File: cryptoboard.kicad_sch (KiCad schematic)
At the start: 27 parts, among them J1 USB_A, J2 BOOT, J3 SWD, SW1 SW_Push, U1 STM32F103C8Tx, U2 LM317_SOT-223-3.3V

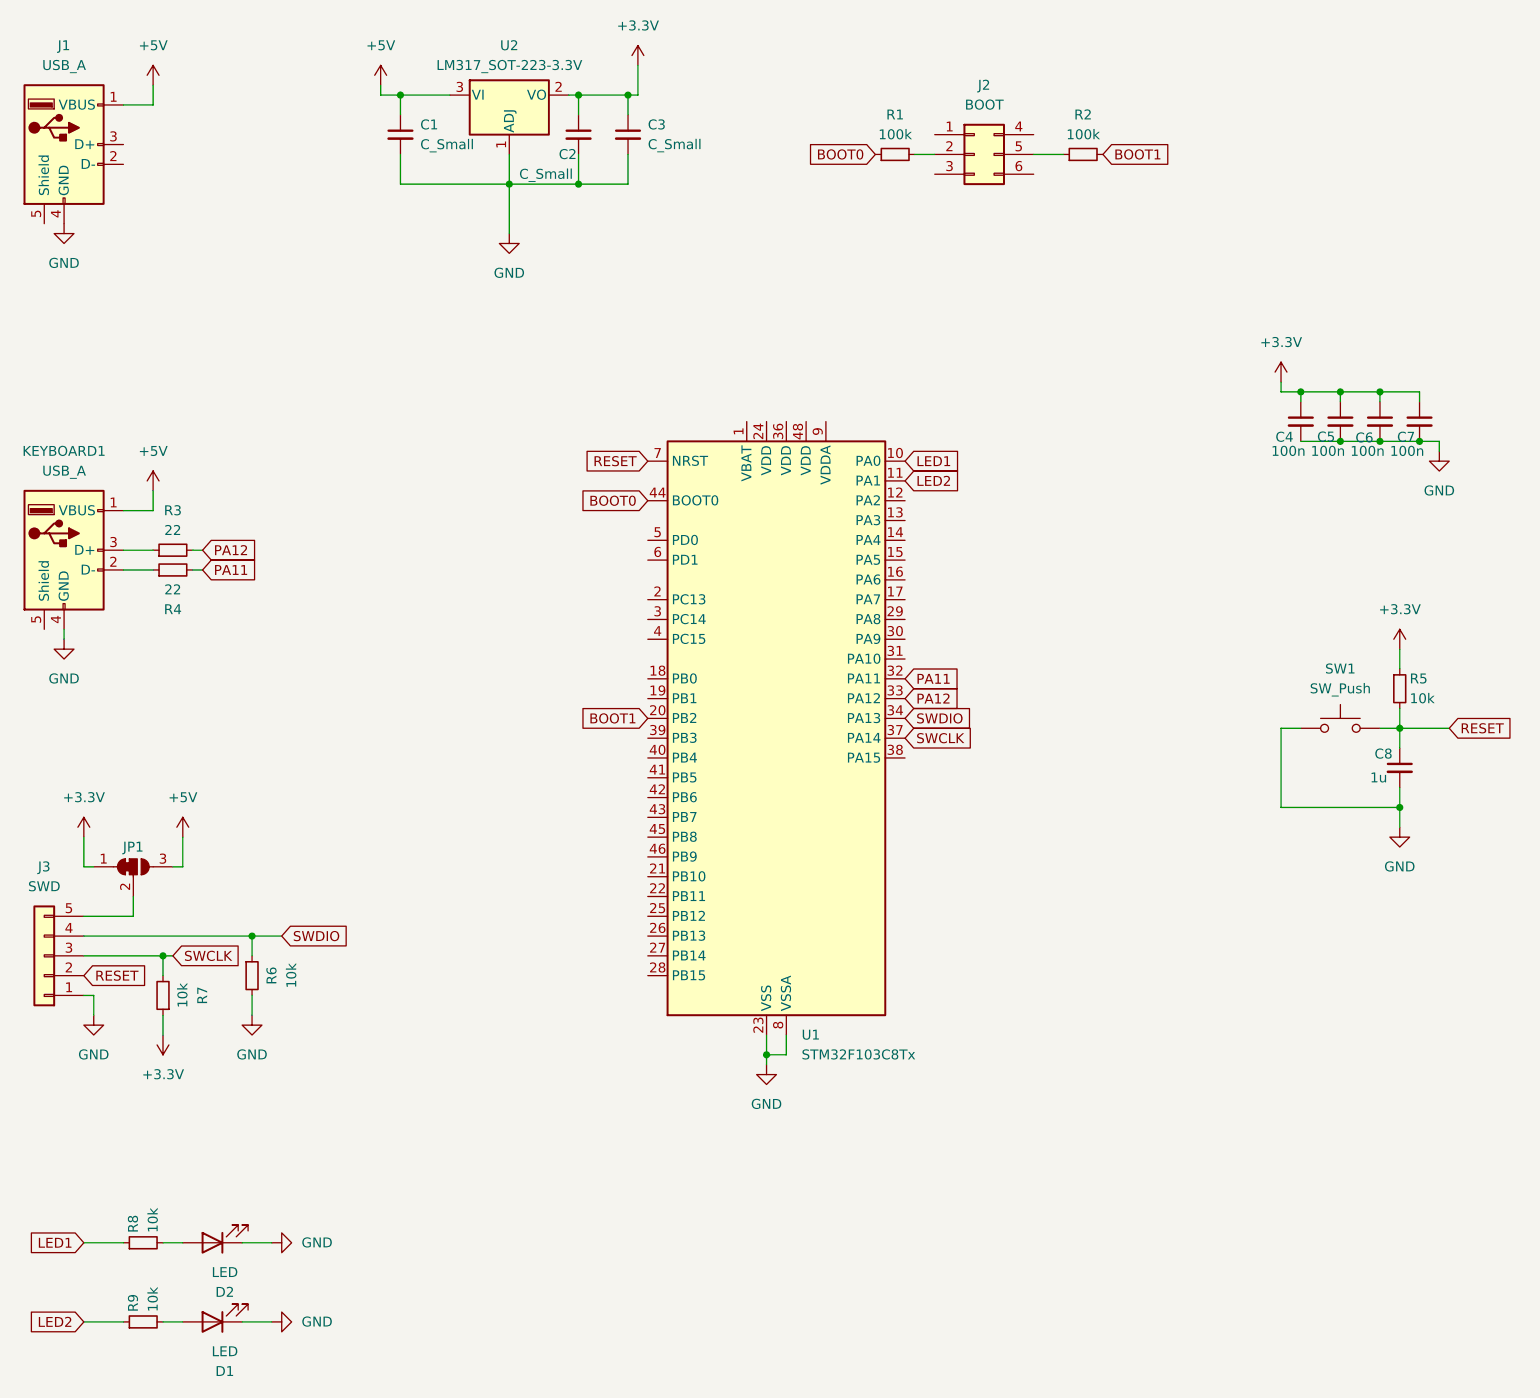
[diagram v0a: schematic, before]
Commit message: add vcc
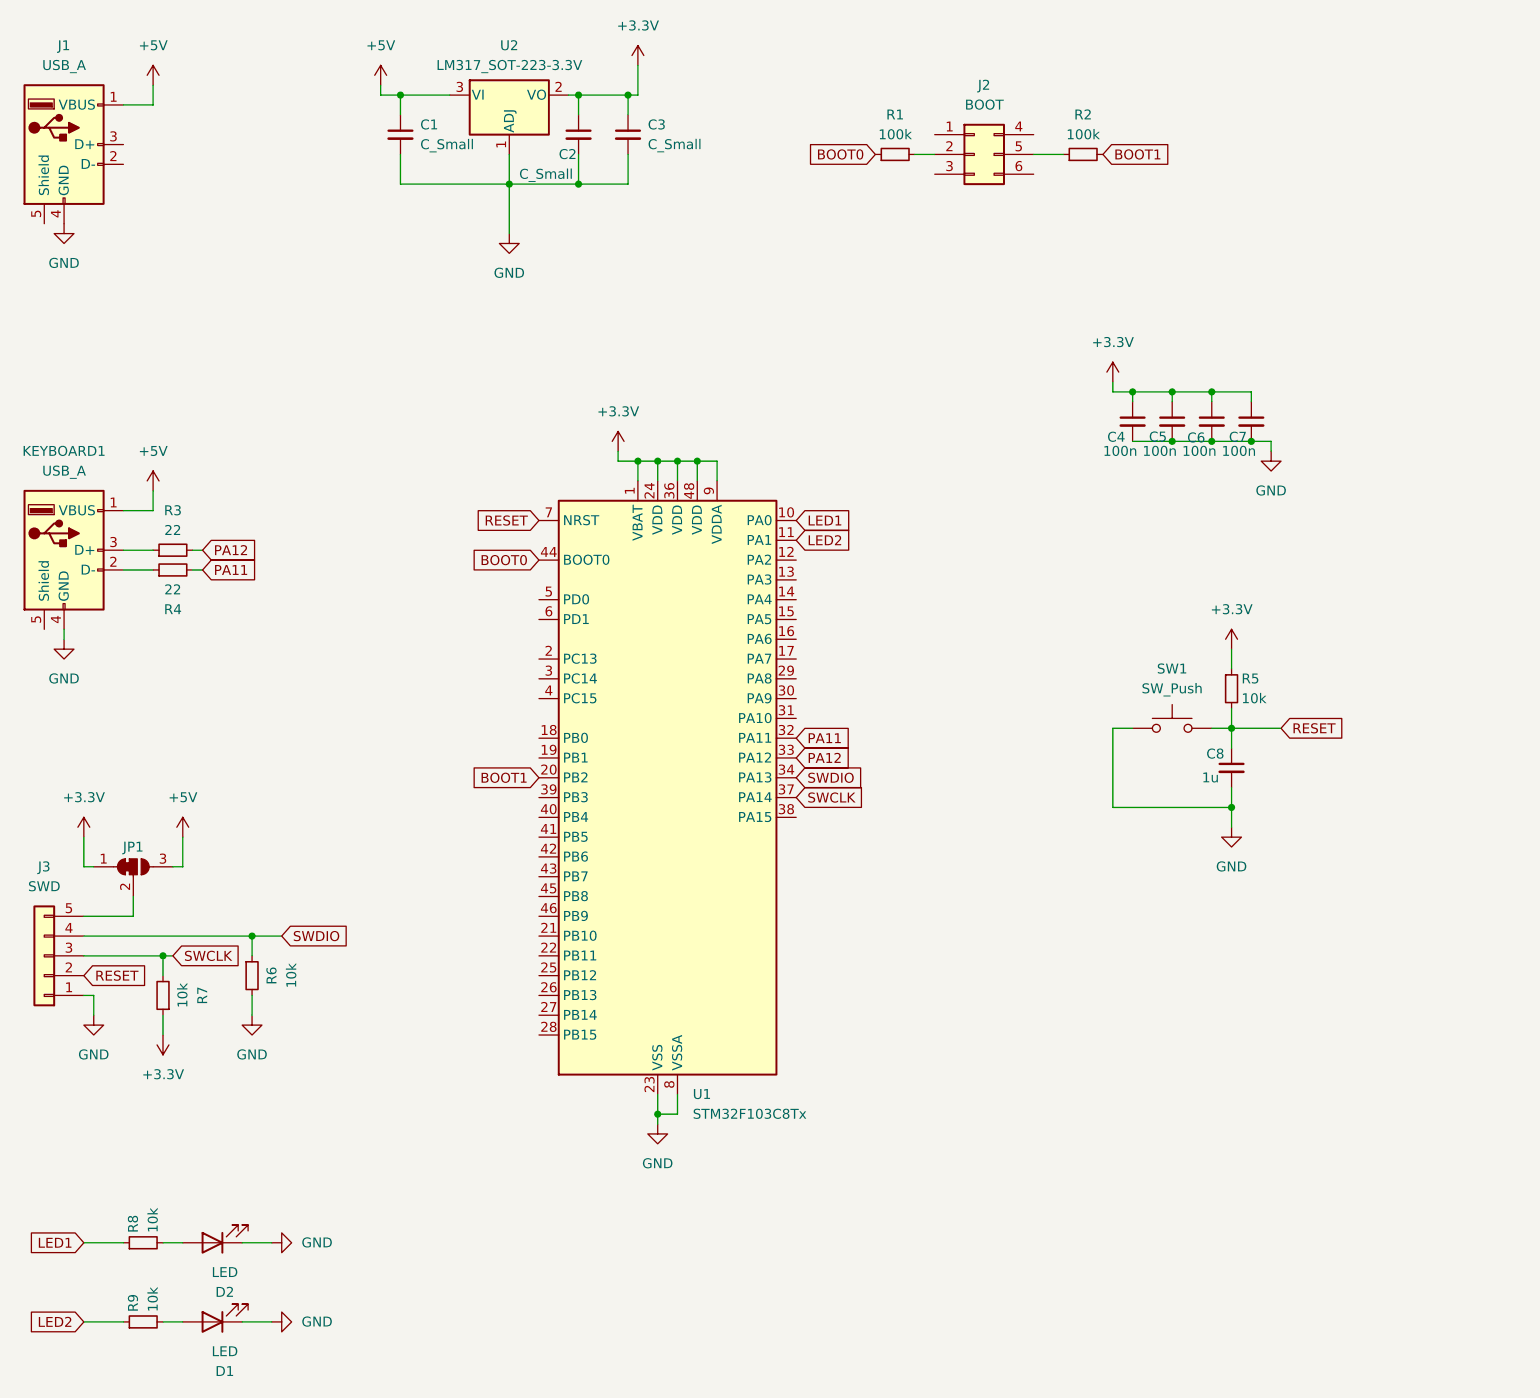
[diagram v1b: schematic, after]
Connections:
- net +3.3V: now also U1.1 (VBAT), U1.24 (VDD), U1.36 (VDD), U1.48 (VDD), U1.9 (VDDA)
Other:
- moved on the sheet: C4, C5, C6, C7, C8, R5, SW1, U1
